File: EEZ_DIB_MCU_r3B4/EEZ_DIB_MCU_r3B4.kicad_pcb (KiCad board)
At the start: 4 copper layers, 139.5 x 70 mm, 119 parts, among them IC1 TPD4E001DRLR, IC11 TPS2051BDBVR, IC12 TPS61169DCKR, IC13 TPD4E001DRLR, IC14 TSC2007IPW, IC2 74AUP1G74DC.125, IC3 CD74HC4050PWR, IC5 LD1117ADT33TR, IC8 AT24C256C-SSHL-B, IC9 N.C., J1 5033981892, J2 67803-8020, J3 HR911130A, J4 Conn_01x22_Socket, Q1 N.C., Q2 2N7002, SW1 TL1100CF160Q, SW2 PEC16-2215F-S0024, U1 ICN6211, X1 DS1024-2*20R0, X2 DS1013-16SSIB1, X3 691322110005

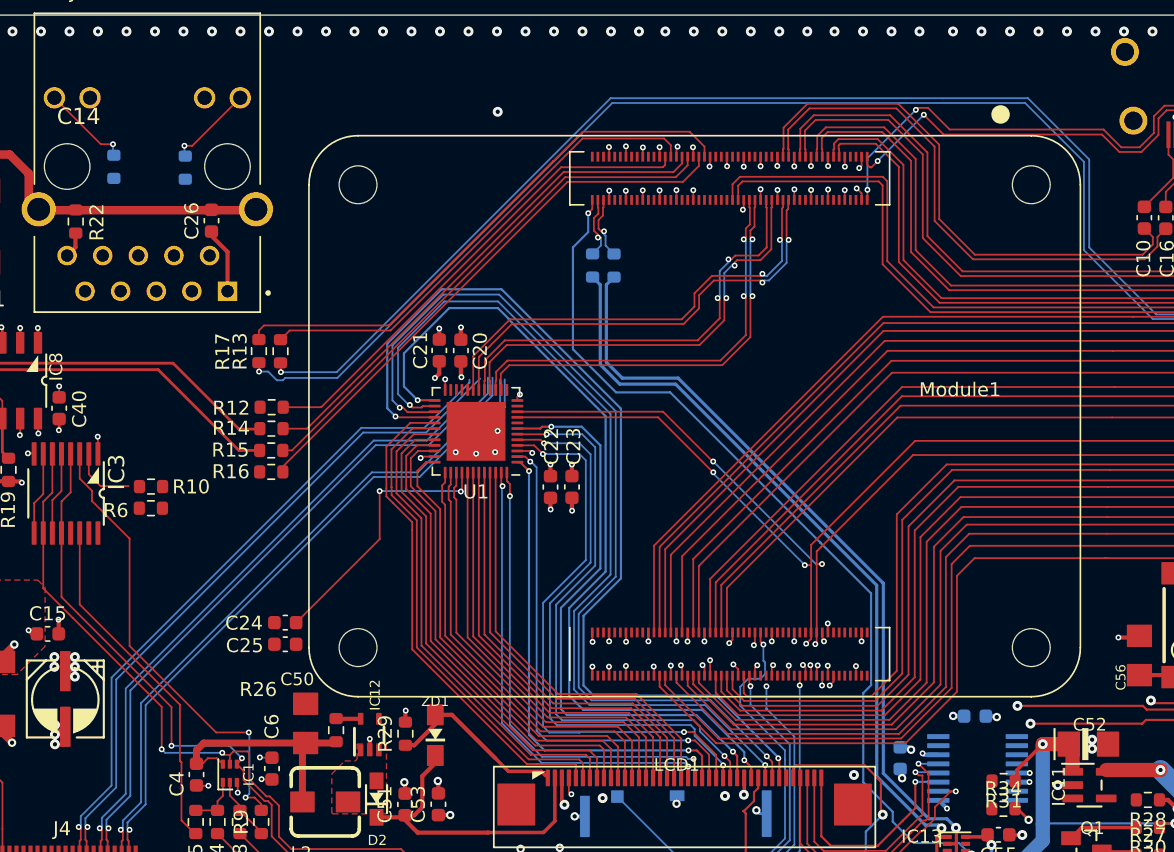
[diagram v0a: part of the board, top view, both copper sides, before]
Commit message: Routing
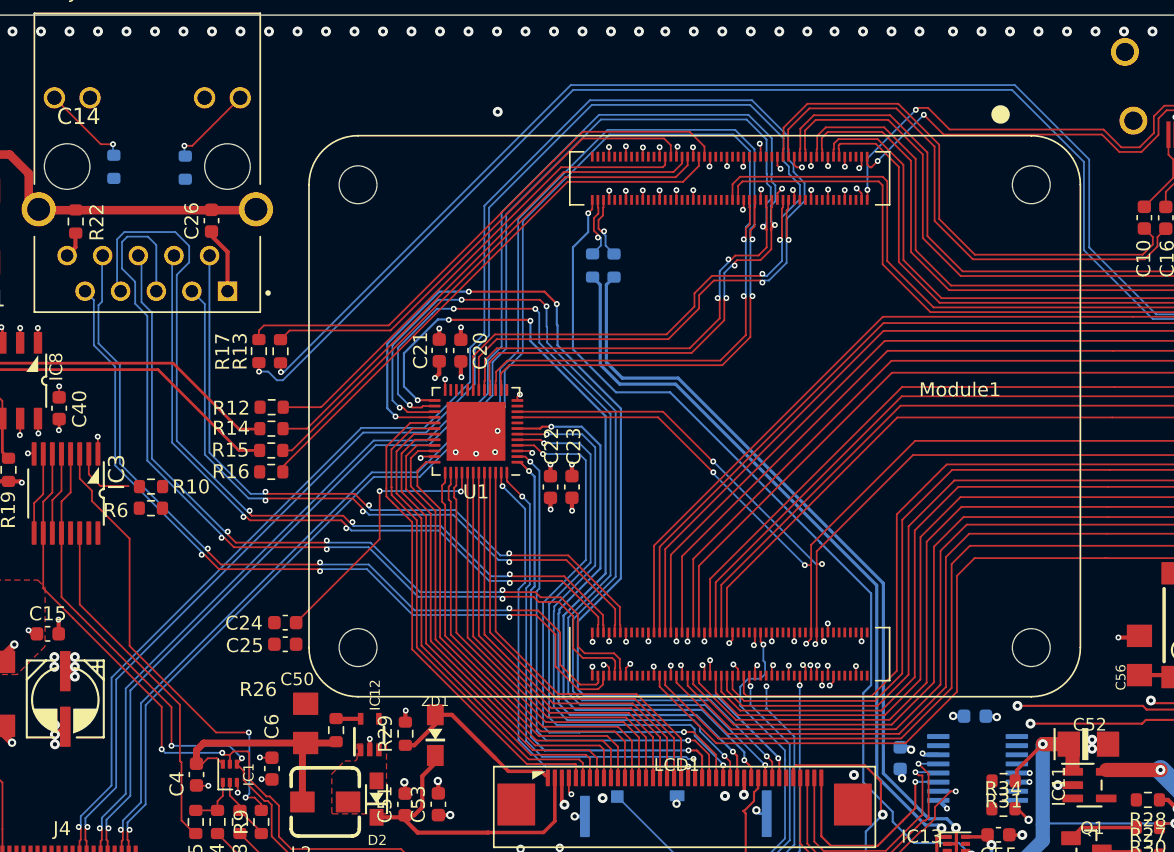
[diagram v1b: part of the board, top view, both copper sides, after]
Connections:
- net /CM4_IO_slow/eth_0n renamed /CM4_IO_slow/ETH_0N
- net /CM4_IO_slow/eth_0p renamed /CM4_IO_slow/ETH_0P
- net /CM4_IO_slow/eth_1n renamed /CM4_IO_slow/ETH_1N
- net /CM4_IO_slow/eth_1p renamed /CM4_IO_slow/ETH_1P
- net /CM4_IO_slow/eth_2n renamed /CM4_IO_slow/ETH_2N
- net /CM4_IO_slow/eth_2p renamed /CM4_IO_slow/ETH_2P
- net /CM4_IO_slow/eth_3n renamed /CM4_IO_slow/ETH_3N
- net /CM4_IO_slow/eth_3p renamed /CM4_IO_slow/ETH_3P
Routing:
- net /CM4_IO_slow/ETH_2P: track 0.00 -> 64.5 mm, vias 0 -> 3
- net /CM4_IO_slow/ETH_1N: track 0.00 -> 61.0 mm, vias 0 -> 3
- net /CM4_IO_slow/ETH_3P: track 0.00 -> 58.5 mm, vias 0 -> 3
- net /CM4_IO_slow/ETH_3N: track 0.00 -> 57.2 mm, vias 0 -> 3
- net /CM4_IO_slow/ETH_2N: track 0.00 -> 57.1 mm, vias 0 -> 3
- net /CM4_IO_slow/ETH_1P: track 0.00 -> 50.4 mm, vias 0 -> 3
- net /CM4_IO_slow/ETH_0P: track 0.00 -> 50.1 mm, vias 0 -> 3
- net /CM4_IO_slow/ETH_0N: track 0.00 -> 47.9 mm, vias 0 -> 3
- net DSIHOST_CKP: track 80.5 -> 127.7 mm
- net DSIHOST_CKN: track 80.8 -> 126.6 mm
- net DSIHOST_D1P: track 79.5 -> 121.6 mm, vias 3 -> 4
- net DSIHOST_D1N: track 79.5 -> 120.5 mm, vias 3 -> 4
- net DSIHOST_D0P: track 78.0 -> 116.6 mm
- net DSIHOST_D0N: track 78.0 -> 115.5 mm
- net LTDC_DE: track 68.4 -> 70.7 mm, vias 2 -> 4
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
